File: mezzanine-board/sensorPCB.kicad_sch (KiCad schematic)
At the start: 22 parts, among them J1 SFMC-105-01-L-D, U1 AS72651, U2 4MB Flash, U3 AS72652, U4 AS72653

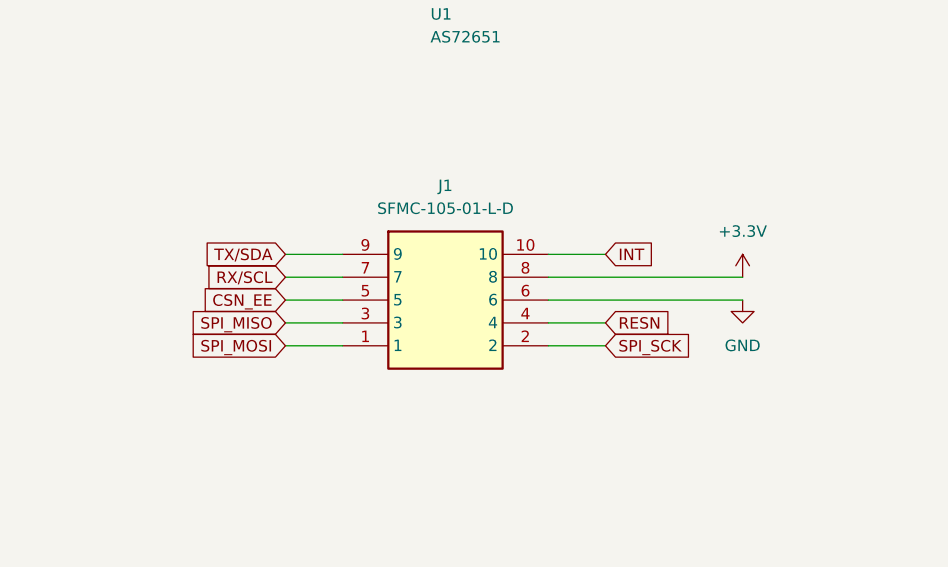
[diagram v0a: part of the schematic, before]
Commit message: Initial Routing
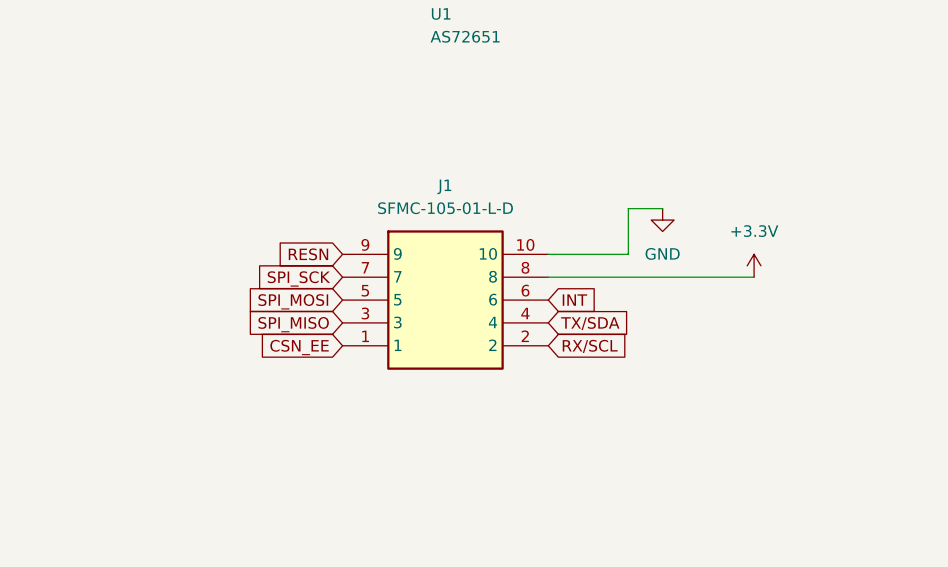
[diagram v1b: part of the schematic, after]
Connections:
- net CSN_EE: now also J1.1; no longer J1.5
- net GND: now also J1.10; no longer J1.6
- net INT: now also J1.6; no longer J1.10
- net RESN: now also J1.9; no longer J1.4
- net RX/SCL: now also J1.2; no longer J1.7
- net SPI_MOSI: now also J1.5; no longer J1.1
- net SPI_SCK: now also J1.7; no longer J1.2
- net TX/SDA: now also J1.4; no longer J1.9
